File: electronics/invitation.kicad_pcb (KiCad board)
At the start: 2 copper layers, 57 x 86 mm, 16 parts, among them P1 USB_OTG, U1 ATMEGA32U4-A, X1 16 MHz

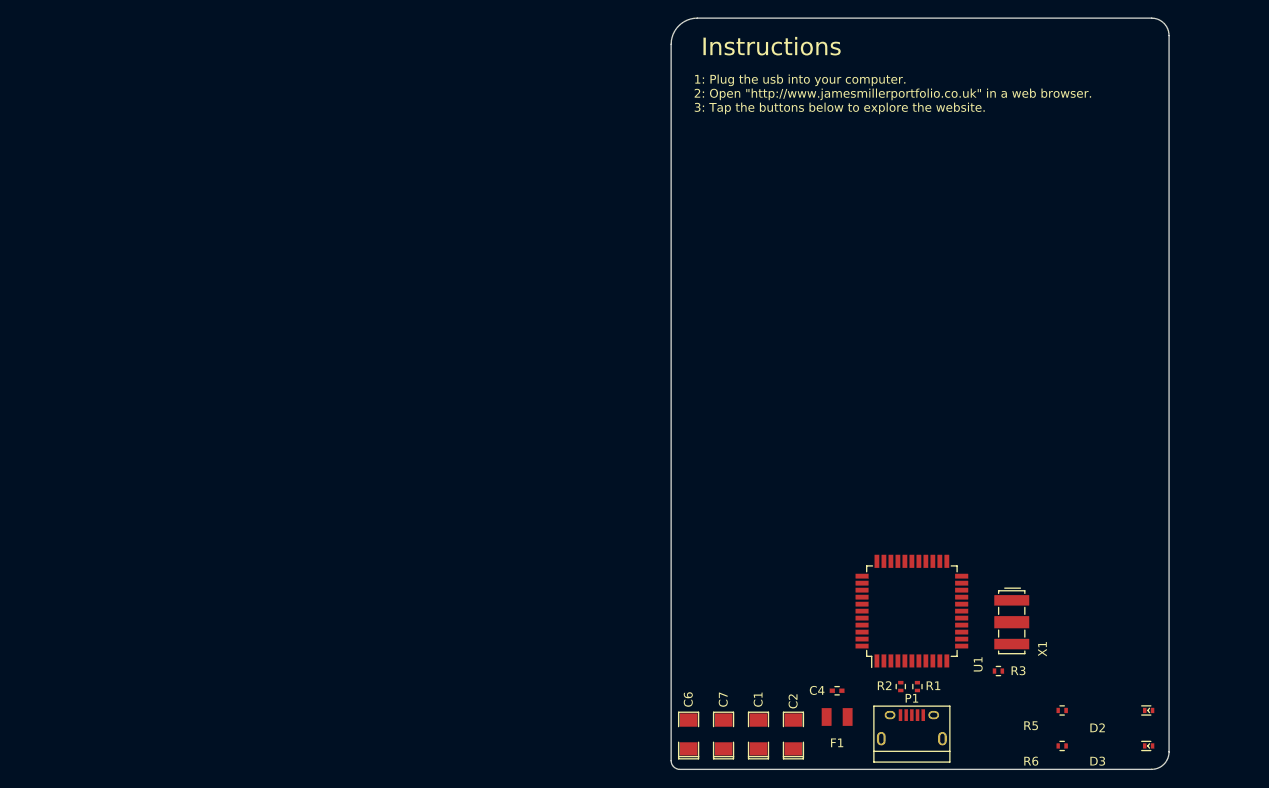
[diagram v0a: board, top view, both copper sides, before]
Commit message: Commit 37: Electronics business card initial design
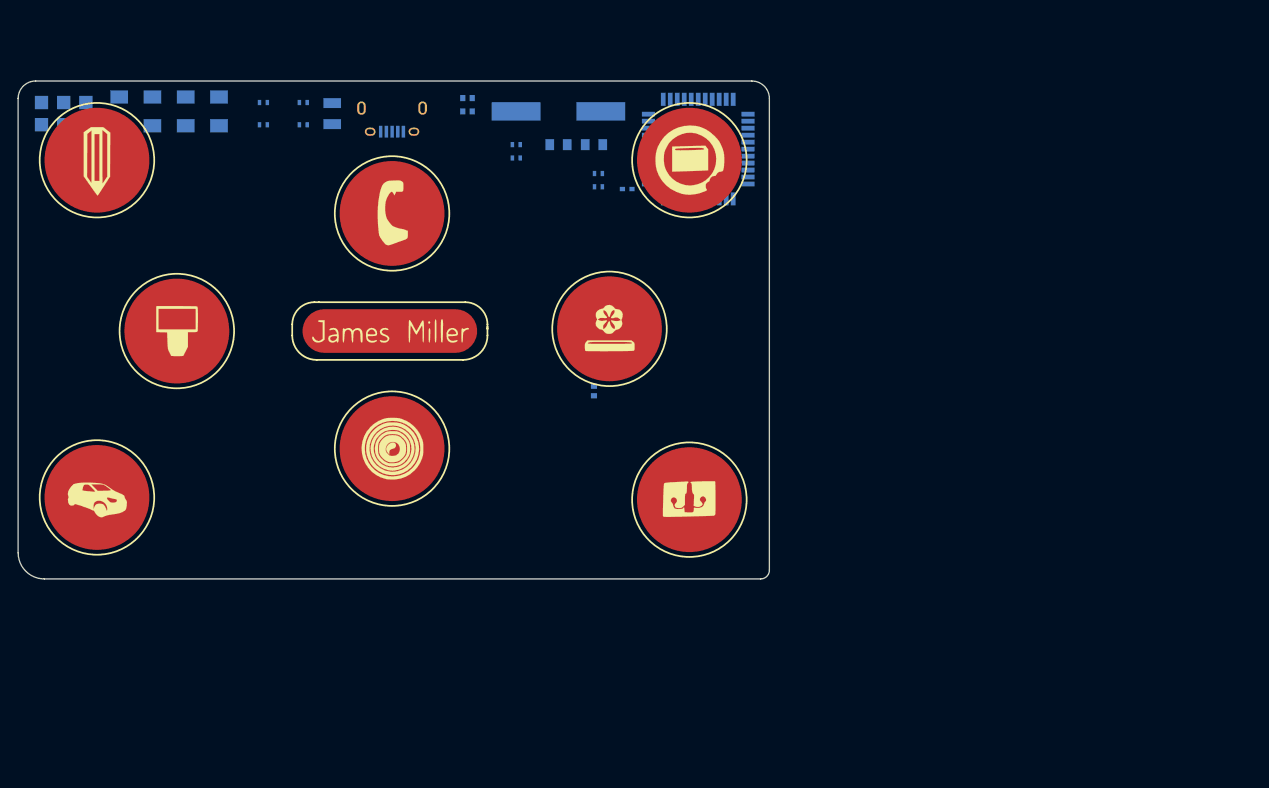
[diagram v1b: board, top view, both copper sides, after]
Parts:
- removed X1: 16 MHz, Crystals:Resonator_7.2x3mm
- added C3: 22pF, Capacitors_SMD:C_0805, B.Cu at (185.2, 78.5)
- added C5: 22pF, Capacitors_SMD:C_0805, B.Cu at (181.1, 78.5)
- added D1: Power LED, LEDs:LED_0402, B.Cu at (185.2, 98.8)
- added D4: TX LED, LEDs:LED_0402, B.Cu at (170.7, 73.2)
- added D5: RX LED, LEDs:LED_0402, B.Cu at (170.7, 74.7)
- added G***: LOGO, assets:mail, B.Cu at (186.2, 124.5)
- added G***: LOGO, assets:phone, B.Cu at (154.2, 124.0)
- added P10: Tassimo, assets:tassimoButton, F.Cu at (186.9, 99.8)
- added P11: Maker, assets:makerButton, F.Cu at (162.1, 113.3)
- added P2: James Miller, assets:JMLogoButton, F.Cu at (162.1, 99.8)
- added P3: CONN_02X03, assets:Programming_port, B.Cu at (127.0, 73.7)
- added P4: D&AD, assets:moodButton, F.Cu at (128.3, 80.3)
- added P5: Krispy Kreme, assets:krispyButton, F.Cu at (196.1, 80.3)
- added P6: Epic Mind Drive, assets:mindDriveButton, F.Cu at (128.3, 119.1)
- added P7: Hacky Xmas, assets:hackyButton, F.Cu at (196.1, 119.1)
- added P8: Pay@Pump, assets:beerButton, F.Cu at (162.1, 86.4)
- added P9: WIYWI, assets:WiywiButton, F.Cu at (137.4, 99.8)
- added R4: 330, Resistors_SMD:R_0402, B.Cu at (147.3, 73.7)
- added R7: 330, Resistors_SMD:R_0402, B.Cu at (151.9, 76.2)
- added R8: 330, Resistors_SMD:R_0402, B.Cu at (147.3, 76.2)
- added Y1: Crystal_Small, Crystals:Crystal_HC49-SD_SMD, B.Cu at (181.1, 74.7)
- C1, C2, C4, C6, C7, F1, P1, R1, R2, R3, R5, R6, U1: moved to B.Cu
- D2: value RX LED -> Interaction LED; moved to B.Cu
- D3: value TX LED -> Node LED; moved to B.Cu
- moved R3 102.8 mm to (151.9, 73.7)
- moved C7 99.4 mm to (130.8, 74.7)
- moved C2 97.0 mm to (142.2, 74.7)
- moved C1 96.9 mm to (138.4, 74.7)
- moved C6 94.1 mm to (134.6, 74.7)
- moved R6 93.0 mm to (176.3, 78.5), turned to 0 degrees
- moved P1 91.8 mm to (162.1, 75.4)
- moved F1 90.1 mm to (155.2, 74.9), turned to 90 degrees
- moved R5 88.9 mm to (176.3, 80.0)
- moved D3 75.4 mm to (185.2, 106.7), turned to 90 degrees
- moved D2 75.3 mm to (185.2, 102.9), turned to 90 degrees
- moved R1 69.2 mm to (185.7, 81.8), turned to 180 degrees
- moved R2 66.9 mm to (185.7, 83.3), turned to 180 degrees
- moved C4 62.3 mm to (189.0, 83.6), turned to 180 degrees
- moved U1 58.3 mm to (197.1, 79.0), turned to 0 degrees
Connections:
- net Net-(R3-Pad1) renamed RESET
- D2 pad 2: VCC -> interactLED
- D3 pad 2: VCC -> nodeLED
- R5 pad 2: Net-(D2-Pad1) -> Net-(D5-Pad1)
- R6 pad 1: Net-(D3-Pad1) -> Net-(D4-Pad1)
- U1 pad 1: Net-(U1-Pad1) -> portfolio5Btn
- U1 pad 10: Net-(U1-Pad10) -> MOSI
- U1 pad 11: Net-(U1-Pad11) -> MISO
- U1 pad 18: Net-(U1-Pad18) -> portfolio2Btn
- U1 pad 19: Net-(U1-Pad19) -> portfolio1Btn
- U1 pad 25: Net-(U1-Pad25) -> portfolio3Btn
- U1 pad 27: Net-(U1-Pad27) -> portfolio4Btn
- U1 pad 28: Net-(U1-Pad28) -> portfolio6Btn
- U1 pad 29: Net-(U1-Pad29) -> nodeLED
- U1 pad 30: Net-(U1-Pad30) -> interactLED
- U1 pad 9: Net-(U1-Pad9) -> SCLK
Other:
- board size 57 x 86 mm -> 86 x 57 mm
- board text added: "+44 (0)7960644904"
- board text added: "Connect this card to your computer using the cable Open in a web browser Tap the buttons below to explore"
- board text added: "How to access James' portfolio:"
- board text added: "info@jamesmillerportfolio.co.uk"
- board text added: "www.jamesmillerportfolio.co.uk"
- board text removed: "1: Plug the usb into your computer. 2: Open "http://www.jamesmillerportfolio.co.uk" in a web browser. 3: Tap the buttons below to explore the website."
- board text removed: "Instructions"
